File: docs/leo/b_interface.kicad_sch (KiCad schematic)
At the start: 8 parts, among them IC37 74LS245, IC38 74LS244, IC39 74LS374, IC40 74LS245, IC46 74LS161, IC47 GAL16V8, IC48 74LS374, IC49 74LS244

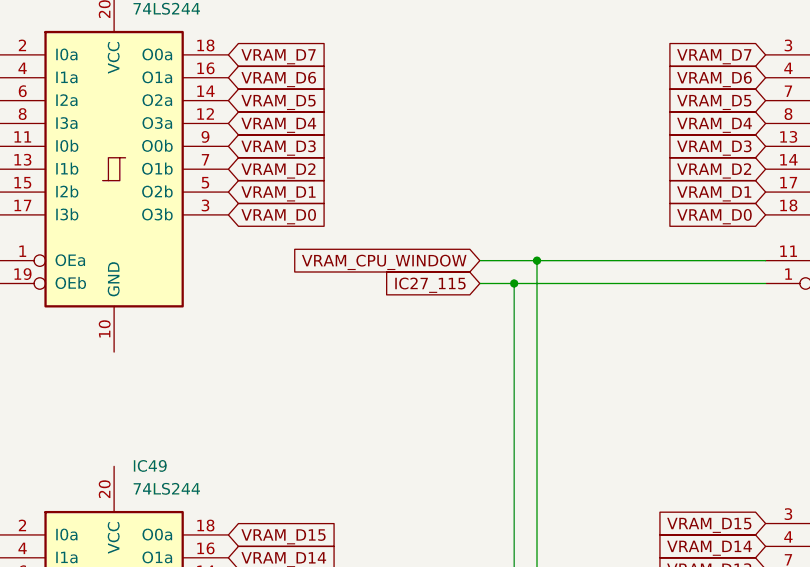
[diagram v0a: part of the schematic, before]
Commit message: Rough out 08J27504
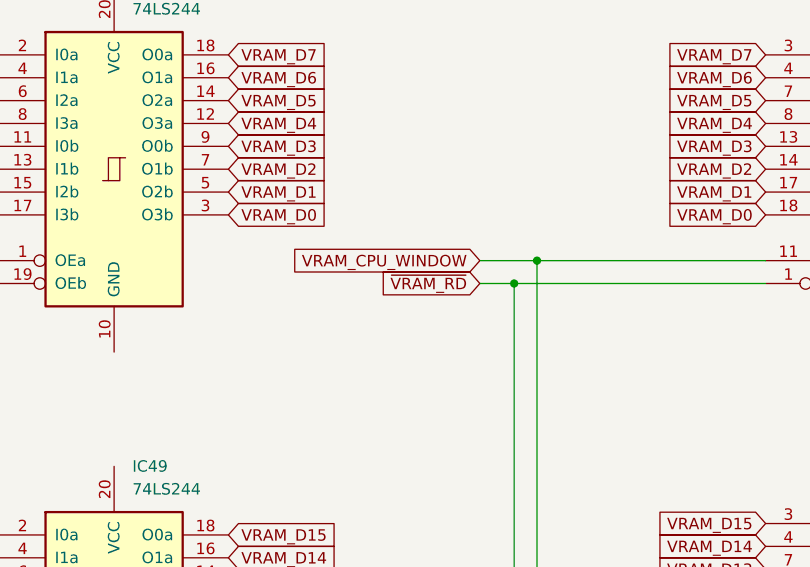
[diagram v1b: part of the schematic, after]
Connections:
- net IC27_115 renamed ~{VRAM_RD}
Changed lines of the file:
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@@
     )
   )
-  (global_label "IC27_115" (shape input) (at 99.06 57.15 180) (fields_autoplaced)
+  (global_label "~{VRAM_RD}" (shape input) (at 99.06 57.15 180) (fields_autoplaced)
     (effects (font (size 1.27 1.27)) (justify right))
-    (property "Intersheet References" "${INTERSHEET_REFS}" (id 0) (at 87.7569 57.0706 0)
+    (property "Intersheet References" "${INTERSHEET_REFS}" (id 0) (at 88.2407 57.0706 0)
       (effects (font (size 1.27 1.27)) (justify right) hide)
     )
